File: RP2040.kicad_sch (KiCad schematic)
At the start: 30 parts, among them J2 Conn_01x02, U18 RP2040, U19 LSF0204PWR, U20 W25Q128JVS, Y1 ABLS-12.000MHZ-B4-T

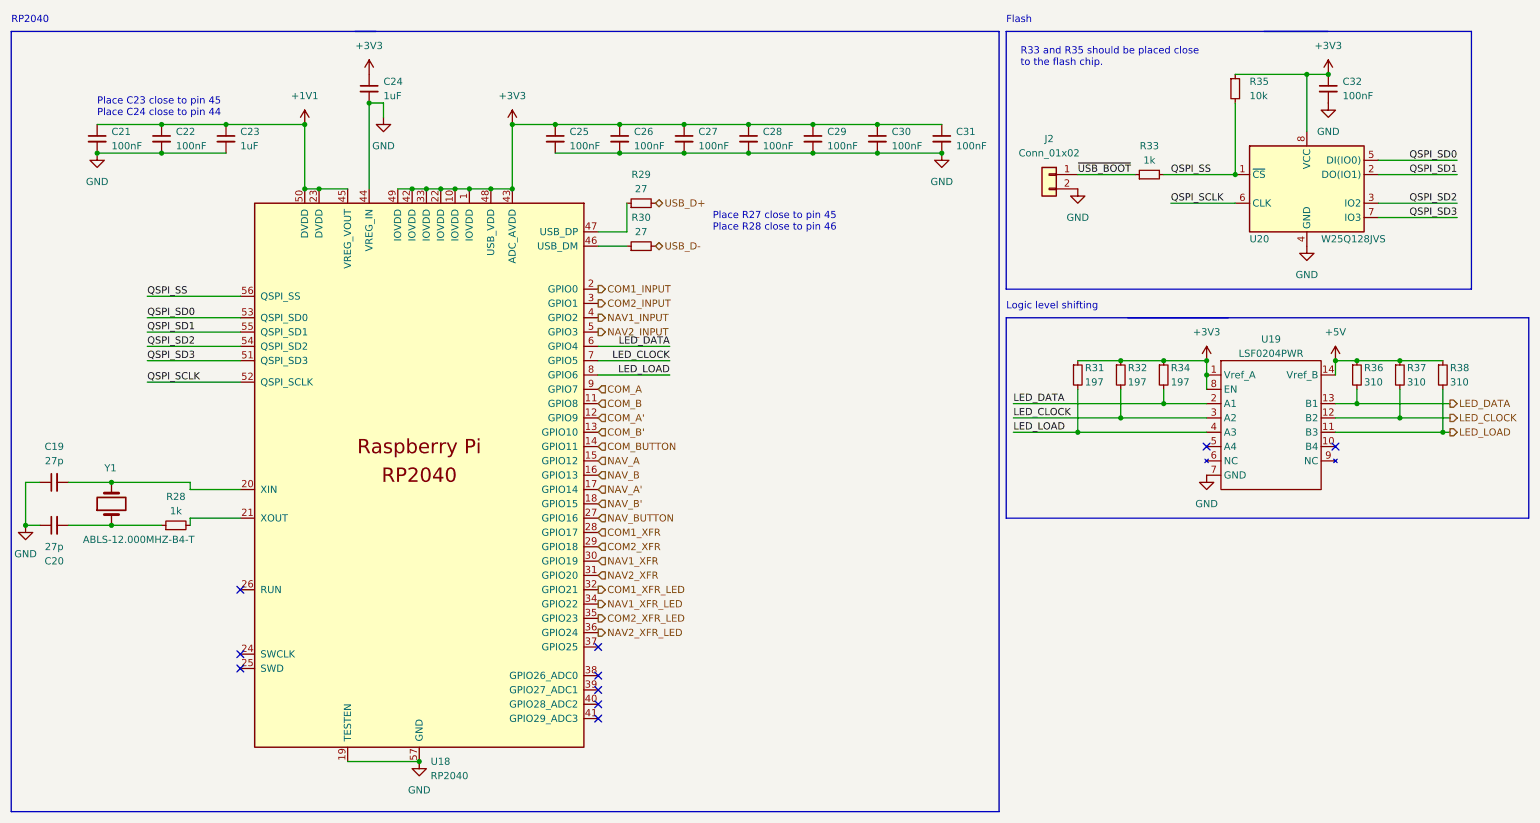
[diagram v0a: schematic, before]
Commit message: Added dual encoder 3d model, fit everything on the board
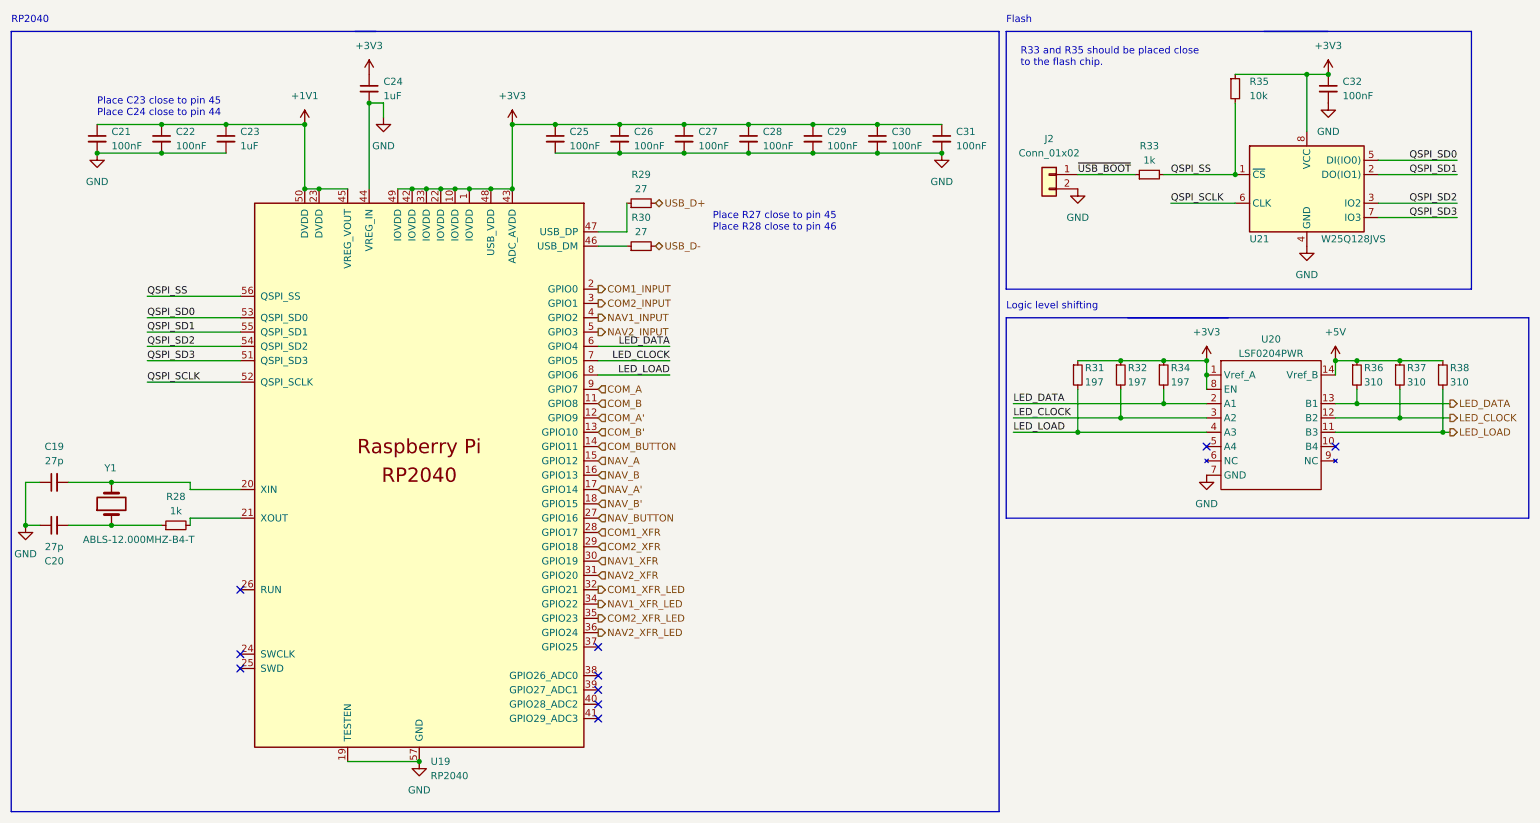
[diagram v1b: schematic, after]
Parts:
- renumbered U18 to U19, U19 to U20, U20 to U21
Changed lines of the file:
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@@
   (symbol (lib_id "power:+3V3") (at 226.06 74.93 0) (unit 1)
     (in_bom yes) (on_board yes) (fields_autoplaced)
-    (property "Reference" "#PWR057" (id 0) (at 226.06 78.74 0)
+    (property "Reference" "#PWR059" (id 0) (at 226.06 78.74 0)
       (effects (font (size 1.27 1.27)) hide)
     )
@@
   (symbol (lib_id "Memory_Flash:W25Q128JVS") (at 243.84 44.45 0) (unit 1)
     (in_bom yes) (on_board yes)
-    (property "Reference" "U20" (id 0) (at 233.68 53.34 0)
+    (property "Reference" "U21" (id 0) (at 233.68 53.34 0)
       (effects (font (size 1.27 1.27)) (justify left))
     )
@@
   (symbol (lib_id "power:+3V3") (at 247.65 24.13 0) (unit 1)
     (in_bom yes) (on_board yes) (fields_autoplaced)
-    (property "Reference" "#PWR060" (id 0) (at 247.65 27.94 0)
+    (property "Reference" "#PWR062" (id 0) (at 247.65 27.94 0)
       (effects (font (size 1.27 1.27)) hide)
     )
@@
   (symbol (lib_id "power:+3V3") (at 102.87 33.02 0) (unit 1)
     (in_bom yes) (on_board yes) (fields_autoplaced)
-    (property "Reference" "#PWR054" (id 0) (at 102.87 36.83 0)
+    (property "Reference" "#PWR056" (id 0) (at 102.87 36.83 0)
       (effects (font (size 1.27 1.27)) hide)
     )
@@
   (symbol (lib_id "power:+1V1") (at 66.04 33.02 0) (unit 1)
     (in_bom yes) (on_board yes) (fields_autoplaced)
-    (property "Reference" "#PWR050" (id 0) (at 66.04 36.83 0)
+    (property "Reference" "#PWR052" (id 0) (at 66.04 36.83 0)
       (effects (font (size 1.27 1.27)) hide)
     )
@@
   (symbol (lib_id "power:GND") (at 29.21 38.1 0) (unit 1)
     (in_bom yes) (on_board yes) (fields_autoplaced)
-    (property "Reference" "#PWR049" (id 0) (at 29.21 44.45 0)
+    (property "Reference" "#PWR051" (id 0) (at 29.21 44.45 0)
       (effects (font (size 1.27 1.27)) hide)
     )
@@
   (symbol (lib_id "power:GND") (at 80.01 31.75 0) (unit 1)
     (in_bom yes) (on_board yes) (fields_autoplaced)
-    (property "Reference" "#PWR052" (id 0) (at 80.01 38.1 0)
+    (property "Reference" "#PWR054" (id 0) (at 80.01 38.1 0)
       (effects (font (size 1.27 1.27)) hide)
     )
@@
   (symbol (lib_id "power:GND") (at 16.51 104.14 0) (unit 1)
     (in_bom yes) (on_board yes) (fields_autoplaced)
-    (property "Reference" "#PWR048" (id 0) (at 16.51 110.49 0)
+    (property "Reference" "#PWR050" (id 0) (at 16.51 110.49 0)
       (effects (font (size 1.27 1.27)) hide)
     )
@@
   (symbol (lib_id "power:GND") (at 243.84 54.61 0) (unit 1)
     (in_bom yes) (on_board yes) (fields_autoplaced)
-    (property "Reference" "#PWR059" (id 0) (at 243.84 60.96 0)
+    (property "Reference" "#PWR061" (id 0) (at 243.84 60.96 0)
       (effects (font (size 1.27 1.27)) hide)
     )
@@
   (symbol (lib_id "power:+5V") (at 248.92 74.93 0) (unit 1)
     (in_bom yes) (on_board yes) (fields_autoplaced)
-    (property "Reference" "#PWR062" (id 0) (at 248.92 78.74 0)
+    (property "Reference" "#PWR064" (id 0) (at 248.92 78.74 0)
       (effects (font (size 1.27 1.27)) hide)
     )
@@
   (symbol (lib_id "Generic-radio-stack:LSF0204PWR") (at 237.49 86.36 0) (unit 1)
     (in_bom yes) (on_board yes)
-    (property "Reference" "U19" (id 0) (at 237.49 71.12 0))
+    (property "Reference" "U20" (id 0) (at 237.49 71.12 0))
     (property "Value" "LSF0204PWR" (id 1) (at 237.49 73.66 0))
     (property "Footprint" "Package_SO:TSSOP-14_4.4x5mm_P0.65mm" (id 2) (at 237.49 102.87 0)
@@
   (symbol (lib_id "power:GND") (at 203.2 44.45 0) (unit 1)
     (in_bom yes) (on_board yes) (fields_autoplaced)
-    (property "Reference" "#PWR056" (id 0) (at 203.2 50.8 0)
+    (property "Reference" "#PWR058" (id 0) (at 203.2 50.8 0)
       (effects (font (size 1.27 1.27)) hide)
     )
@@
   (symbol (lib_id "power:GND") (at 247.65 29.21 0) (unit 1)
     (in_bom yes) (on_board yes) (fields_autoplaced)
-    (property "Reference" "#PWR061" (id 0) (at 247.65 35.56 0)
+    (property "Reference" "#PWR063" (id 0) (at 247.65 35.56 0)
       (effects (font (size 1.27 1.27)) hide)
     )
@@
   (symbol (lib_id "power:+3V3") (at 77.47 24.13 0) (unit 1)
     (in_bom yes) (on_board yes) (fields_autoplaced)
-    (property "Reference" "#PWR051" (id 0) (at 77.47 27.94 0)
+    (property "Reference" "#PWR053" (id 0) (at 77.47 27.94 0)
       (effects (font (size 1.27 1.27)) hide)
     )
@@
   (symbol (lib_id "power:GND") (at 226.06 95.25 0) (unit 1)
     (in_bom yes) (on_board yes) (fields_autoplaced)
-    (property "Reference" "#PWR058" (id 0) (at 226.06 101.6 0)
+    (property "Reference" "#PWR060" (id 0) (at 226.06 101.6 0)
       (effects (font (size 1.27 1.27)) hide)
     )
@@
   (symbol (lib_id "power:GND") (at 179.07 38.1 0) (unit 1)
     (in_bom yes) (on_board yes) (fields_autoplaced)
-    (property "Reference" "#PWR055" (id 0) (at 179.07 44.45 0)
+    (property "Reference" "#PWR057" (id 0) (at 179.07 44.45 0)
       (effects (font (size 1.27 1.27)) hide)
     )
@@
   (symbol (lib_id "MCU_RaspberryPi_RP2040:RP2040") (at 86.36 95.25 0) (unit 1)
     (in_bom yes) (on_board yes) (fields_autoplaced)
-    (property "Reference" "U18" (id 0) (at 88.3794 146.05 0)
+    (property "Reference" "U19" (id 0) (at 88.3794 146.05 0)
       (effects (font (size 1.27 1.27)) (justify left))
     )
@@
   (symbol (lib_id "power:GND") (at 86.36 146.05 0) (unit 1)
     (in_bom yes) (on_board yes) (fields_autoplaced)
-    (property "Reference" "#PWR053" (id 0) (at 86.36 152.4 0)
-      (effects (font (size 1.27 1.27)) hide)
-    )
+    (property "Reference" "#PWR055" (id 0) (at 86.36 152.4 0)
+      (effects (font (size 1.27 1.27)) hide)
+    )

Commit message: Add mounting holes
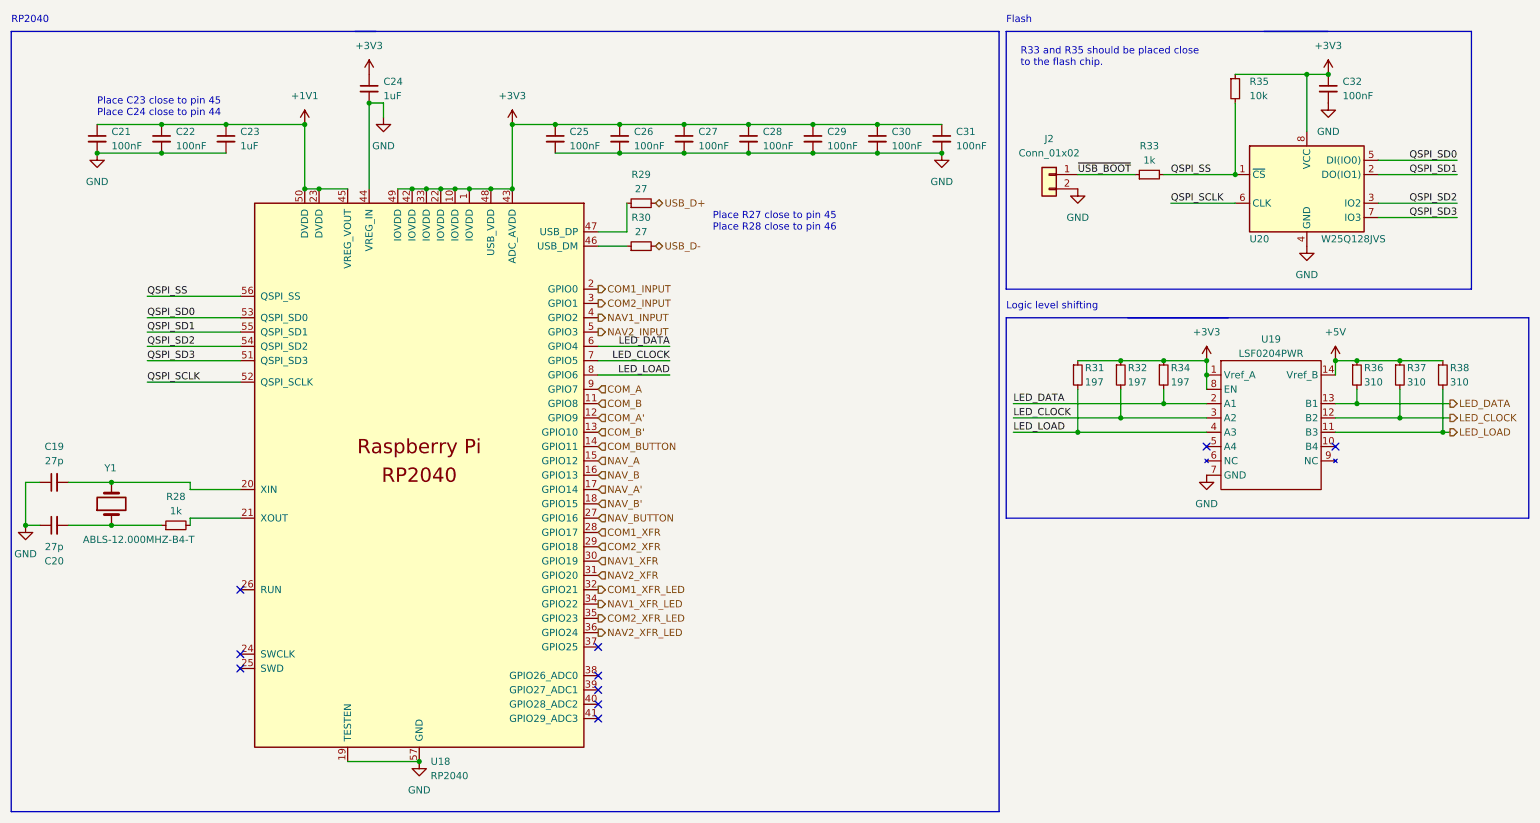
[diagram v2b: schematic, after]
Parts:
- renumbered U19 to U18, U20 to U19, U21 to U20
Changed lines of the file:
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@@
   (symbol (lib_id "power:+3V3") (at 226.06 74.93 0) (unit 1)
     (in_bom yes) (on_board yes) (fields_autoplaced)
-    (property "Reference" "#PWR059" (id 0) (at 226.06 78.74 0)
+    (property "Reference" "#PWR057" (id 0) (at 226.06 78.74 0)
       (effects (font (size 1.27 1.27)) hide)
     )
@@
   (symbol (lib_id "Memory_Flash:W25Q128JVS") (at 243.84 44.45 0) (unit 1)
     (in_bom yes) (on_board yes)
-    (property "Reference" "U21" (id 0) (at 233.68 53.34 0)
+    (property "Reference" "U20" (id 0) (at 233.68 53.34 0)
       (effects (font (size 1.27 1.27)) (justify left))
     )
@@
   (symbol (lib_id "power:+3V3") (at 247.65 24.13 0) (unit 1)
     (in_bom yes) (on_board yes) (fields_autoplaced)
-    (property "Reference" "#PWR062" (id 0) (at 247.65 27.94 0)
+    (property "Reference" "#PWR060" (id 0) (at 247.65 27.94 0)
       (effects (font (size 1.27 1.27)) hide)
     )
@@
   (symbol (lib_id "power:+3V3") (at 102.87 33.02 0) (unit 1)
     (in_bom yes) (on_board yes) (fields_autoplaced)
-    (property "Reference" "#PWR056" (id 0) (at 102.87 36.83 0)
+    (property "Reference" "#PWR054" (id 0) (at 102.87 36.83 0)
       (effects (font (size 1.27 1.27)) hide)
     )
@@
   (symbol (lib_id "power:+1V1") (at 66.04 33.02 0) (unit 1)
     (in_bom yes) (on_board yes) (fields_autoplaced)
-    (property "Reference" "#PWR052" (id 0) (at 66.04 36.83 0)
+    (property "Reference" "#PWR050" (id 0) (at 66.04 36.83 0)
       (effects (font (size 1.27 1.27)) hide)
     )
@@
   (symbol (lib_id "power:GND") (at 29.21 38.1 0) (unit 1)
     (in_bom yes) (on_board yes) (fields_autoplaced)
-    (property "Reference" "#PWR051" (id 0) (at 29.21 44.45 0)
+    (property "Reference" "#PWR049" (id 0) (at 29.21 44.45 0)
       (effects (font (size 1.27 1.27)) hide)
     )
@@
   (symbol (lib_id "power:GND") (at 80.01 31.75 0) (unit 1)
     (in_bom yes) (on_board yes) (fields_autoplaced)
-    (property "Reference" "#PWR054" (id 0) (at 80.01 38.1 0)
+    (property "Reference" "#PWR052" (id 0) (at 80.01 38.1 0)
       (effects (font (size 1.27 1.27)) hide)
     )
@@
   (symbol (lib_id "power:GND") (at 16.51 104.14 0) (unit 1)
     (in_bom yes) (on_board yes) (fields_autoplaced)
-    (property "Reference" "#PWR050" (id 0) (at 16.51 110.49 0)
+    (property "Reference" "#PWR048" (id 0) (at 16.51 110.49 0)
       (effects (font (size 1.27 1.27)) hide)
     )
@@
   (symbol (lib_id "power:GND") (at 243.84 54.61 0) (unit 1)
     (in_bom yes) (on_board yes) (fields_autoplaced)
-    (property "Reference" "#PWR061" (id 0) (at 243.84 60.96 0)
+    (property "Reference" "#PWR059" (id 0) (at 243.84 60.96 0)
       (effects (font (size 1.27 1.27)) hide)
     )
@@
   (symbol (lib_id "power:+5V") (at 248.92 74.93 0) (unit 1)
     (in_bom yes) (on_board yes) (fields_autoplaced)
-    (property "Reference" "#PWR064" (id 0) (at 248.92 78.74 0)
+    (property "Reference" "#PWR062" (id 0) (at 248.92 78.74 0)
       (effects (font (size 1.27 1.27)) hide)
     )
@@
   (symbol (lib_id "Generic-radio-stack:LSF0204PWR") (at 237.49 86.36 0) (unit 1)
     (in_bom yes) (on_board yes)
-    (property "Reference" "U20" (id 0) (at 237.49 71.12 0))
+    (property "Reference" "U19" (id 0) (at 237.49 71.12 0))
     (property "Value" "LSF0204PWR" (id 1) (at 237.49 73.66 0))
     (property "Footprint" "Package_SO:TSSOP-14_4.4x5mm_P0.65mm" (id 2) (at 237.49 102.87 0)
@@
   (symbol (lib_id "power:GND") (at 203.2 44.45 0) (unit 1)
     (in_bom yes) (on_board yes) (fields_autoplaced)
-    (property "Reference" "#PWR058" (id 0) (at 203.2 50.8 0)
+    (property "Reference" "#PWR056" (id 0) (at 203.2 50.8 0)
       (effects (font (size 1.27 1.27)) hide)
     )
@@
   (symbol (lib_id "power:GND") (at 247.65 29.21 0) (unit 1)
     (in_bom yes) (on_board yes) (fields_autoplaced)
-    (property "Reference" "#PWR063" (id 0) (at 247.65 35.56 0)
+    (property "Reference" "#PWR061" (id 0) (at 247.65 35.56 0)
       (effects (font (size 1.27 1.27)) hide)
     )
@@
   (symbol (lib_id "power:+3V3") (at 77.47 24.13 0) (unit 1)
     (in_bom yes) (on_board yes) (fields_autoplaced)
-    (property "Reference" "#PWR053" (id 0) (at 77.47 27.94 0)
+    (property "Reference" "#PWR051" (id 0) (at 77.47 27.94 0)
       (effects (font (size 1.27 1.27)) hide)
     )
@@
   (symbol (lib_id "power:GND") (at 226.06 95.25 0) (unit 1)
     (in_bom yes) (on_board yes) (fields_autoplaced)
-    (property "Reference" "#PWR060" (id 0) (at 226.06 101.6 0)
+    (property "Reference" "#PWR058" (id 0) (at 226.06 101.6 0)
       (effects (font (size 1.27 1.27)) hide)
     )
@@
   (symbol (lib_id "power:GND") (at 179.07 38.1 0) (unit 1)
     (in_bom yes) (on_board yes) (fields_autoplaced)
-    (property "Reference" "#PWR057" (id 0) (at 179.07 44.45 0)
+    (property "Reference" "#PWR055" (id 0) (at 179.07 44.45 0)
       (effects (font (size 1.27 1.27)) hide)
     )
@@
   (symbol (lib_id "MCU_RaspberryPi_RP2040:RP2040") (at 86.36 95.25 0) (unit 1)
     (in_bom yes) (on_board yes) (fields_autoplaced)
-    (property "Reference" "U19" (id 0) (at 88.3794 146.05 0)
+    (property "Reference" "U18" (id 0) (at 88.3794 146.05 0)
       (effects (font (size 1.27 1.27)) (justify left))
     )
@@
   (symbol (lib_id "power:GND") (at 86.36 146.05 0) (unit 1)
     (in_bom yes) (on_board yes) (fields_autoplaced)
-    (property "Reference" "#PWR055" (id 0) (at 86.36 152.4 0)
-      (effects (font (size 1.27 1.27)) hide)
-    )
+    (property "Reference" "#PWR053" (id 0) (at 86.36 152.4 0)
+      (effects (font (size 1.27 1.27)) hide)
+    )
